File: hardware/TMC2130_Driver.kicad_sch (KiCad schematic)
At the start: 35 parts, among them J1 PCIe_Stepper, J2 Conn_01x04_Male, J3 Screw_Terminal_01x02, U1 TMC2130, U2 24LC02

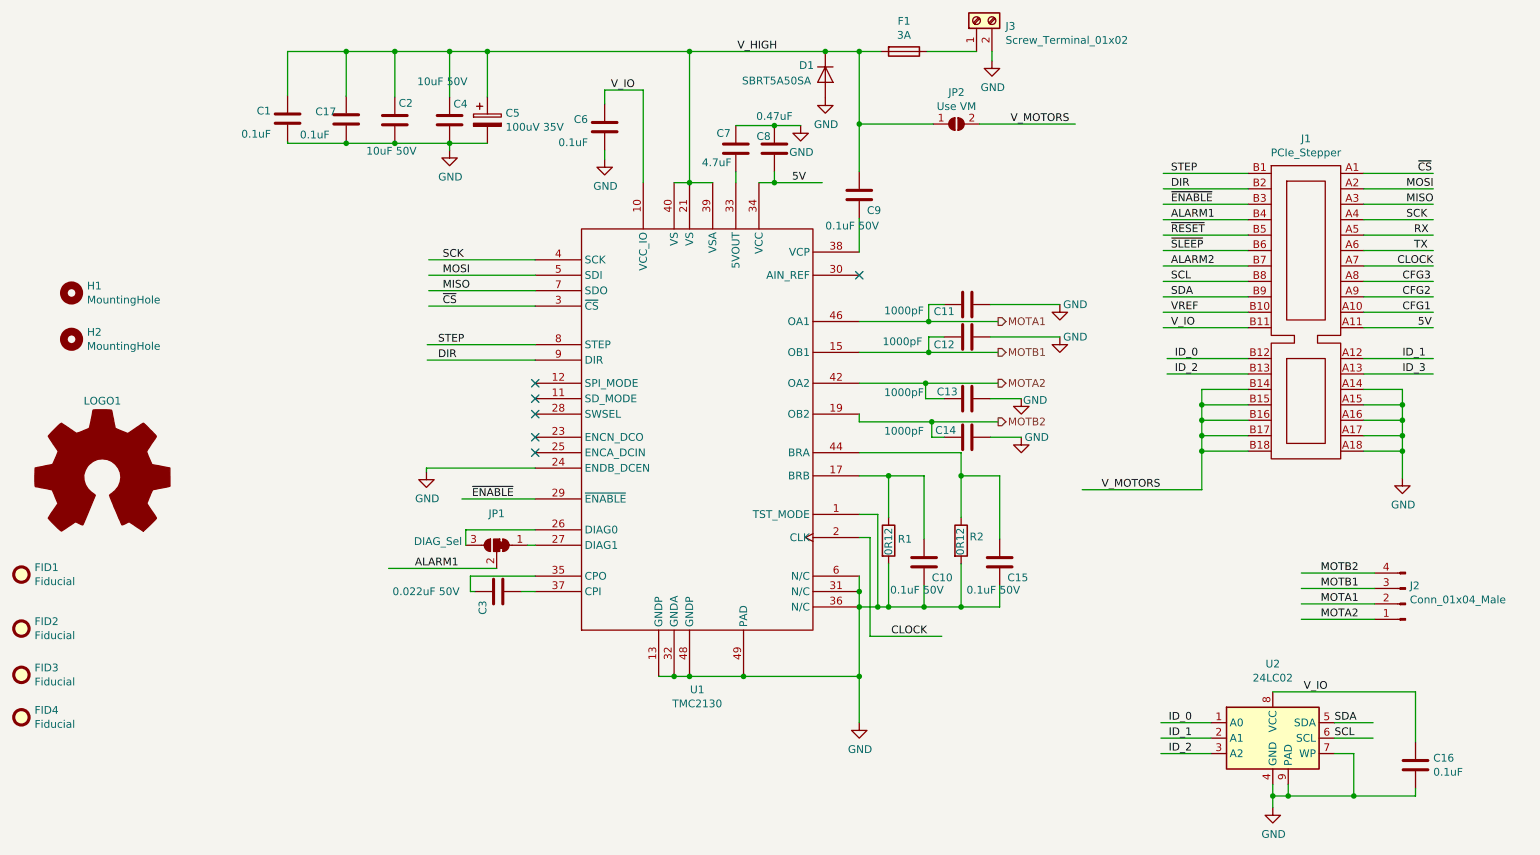
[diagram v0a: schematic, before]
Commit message: Update 2660 and 2130 driver fab files.
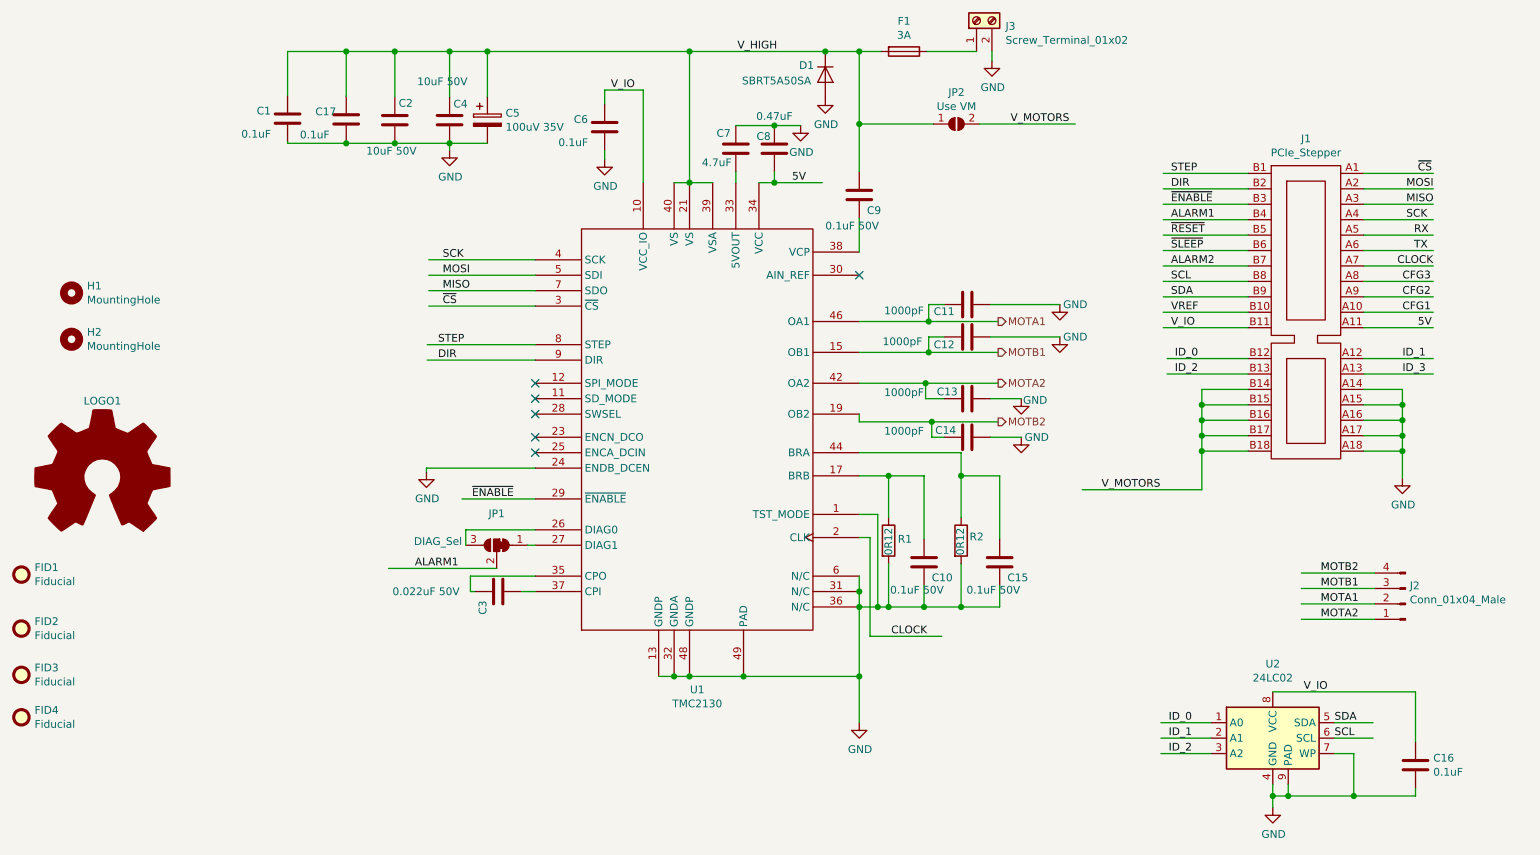
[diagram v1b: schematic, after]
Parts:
- FID1, FID2, FID3, FID4, H1, H2, LOGO1: now left out of the parts list
- U2: LCSC Part # C184154 -> C184154
